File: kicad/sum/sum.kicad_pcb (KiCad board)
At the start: 2 copper layers, 69 x 46 mm, 18 parts

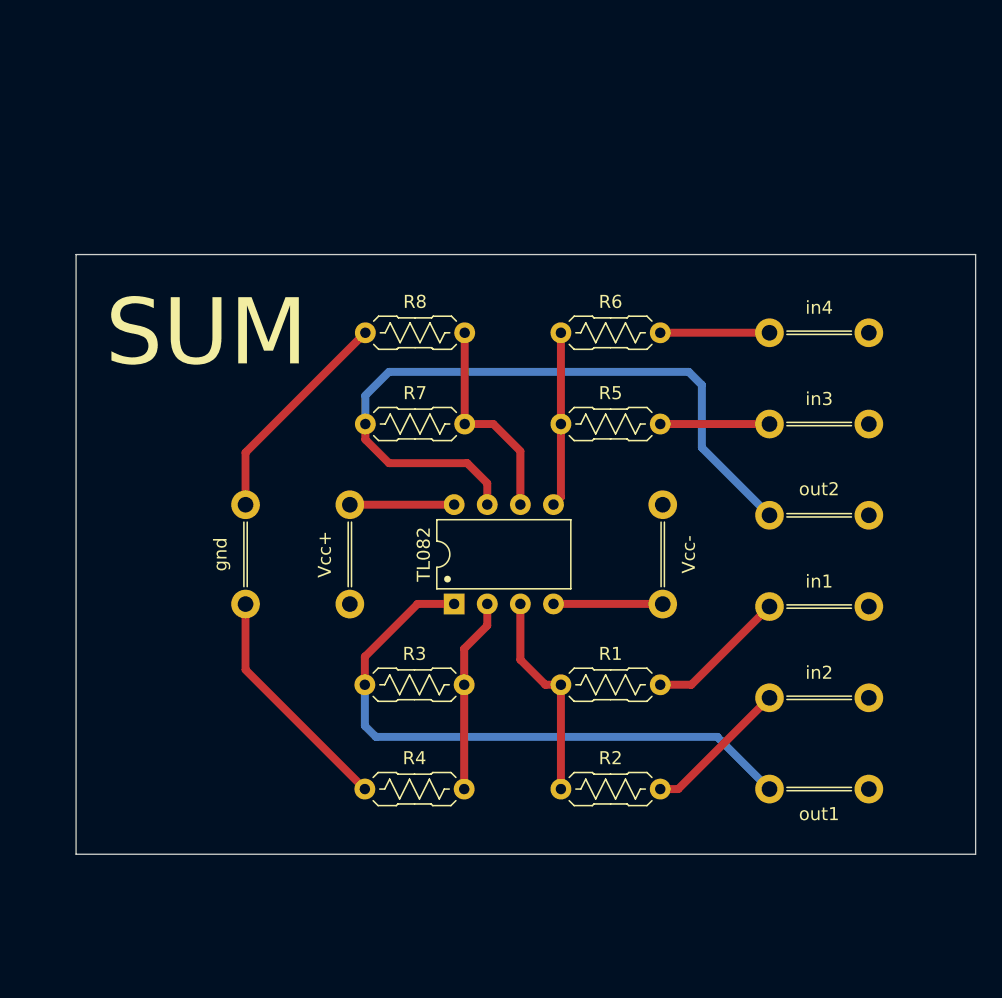
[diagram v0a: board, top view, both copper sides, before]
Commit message: Add files via upload
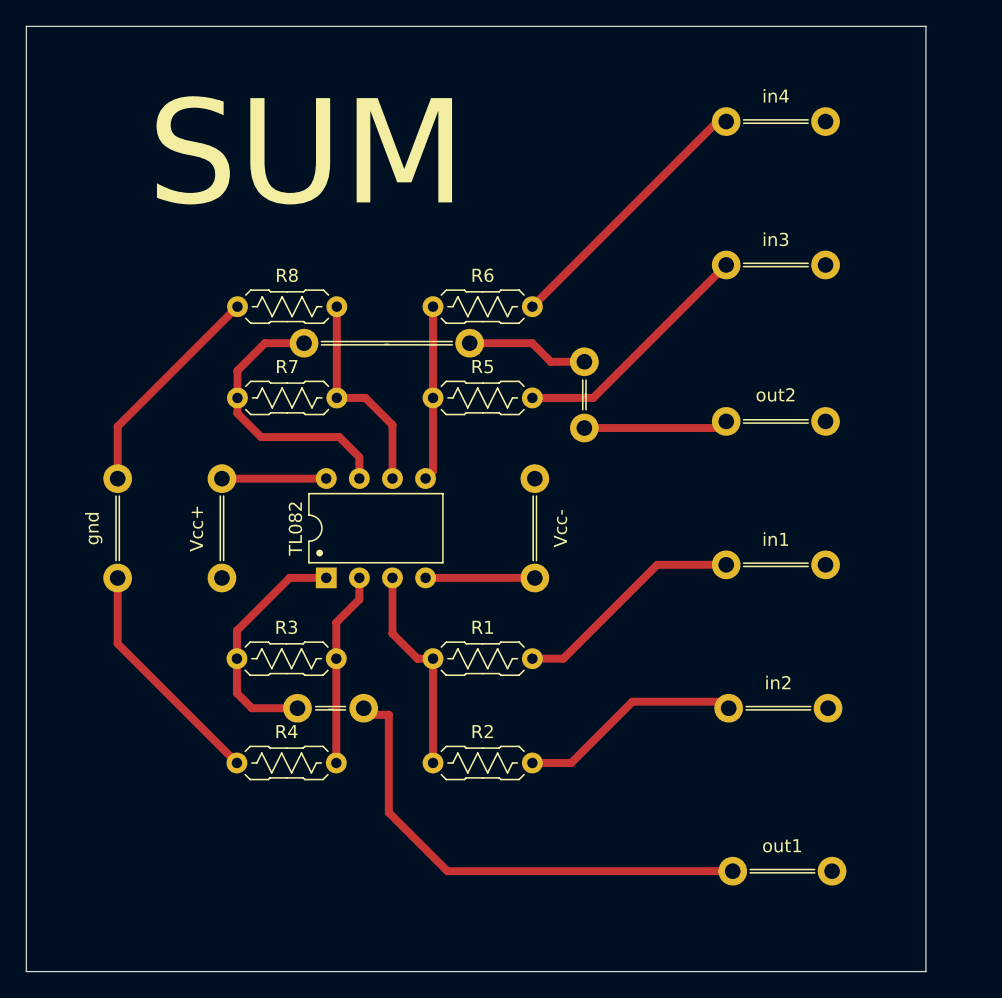
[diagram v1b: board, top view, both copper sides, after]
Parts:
- added -: Jumper_P5.08mm_D1.2mm, PCM_Jumper_AKL:Jumper_P5.08mm_D1.2mm, F.Cu at (147.0, 93.5)
- added -: Jumper_P12.70mm_D1.2mm, PCM_Jumper_AKL:Jumper_P12.70mm_D1.2mm, F.Cu at (125.5, 87.0)
- added -: Jumper_P5.08mm_D1.2mm, PCM_Jumper_AKL:Jumper_P5.08mm_D1.2mm, F.Cu at (125.0, 115.0)
- moved in4 16.5 mm to (157.9, 70.0)
- moved in3 12.6 mm to (157.9, 81.0)
- moved out1 12.2 mm to (158.4, 127.5), turned to 0 degrees
- moved R1 10.0 mm to (135.4, 111.2)
- moved R2 10.0 mm to (135.4, 119.2)
- moved R3 10.0 mm to (120.4, 111.2)
- moved R4 10.0 mm to (120.4, 119.2)
- moved R5 10.0 mm to (135.4, 91.2)
- moved R6 10.0 mm to (135.4, 84.2)
- moved Vcc- 10.0 mm to (143.2, 105.0)
- moved gnd 10.0 mm to (111.2, 105.0)
- moved R7 10.0 mm to (120.4, 91.2)
- moved R8 10.0 mm to (120.4, 84.2)
- moved TL082 10.0 mm to (127.2, 105.0)
- moved Vcc+ 10.0 mm to (119.2, 105.0)
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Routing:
- net (no net): track 252.8 -> 285.3 mm
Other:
- board size 69 x 46 mm -> 69 x 72.5 mm
